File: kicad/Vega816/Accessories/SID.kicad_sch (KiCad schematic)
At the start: 18 parts

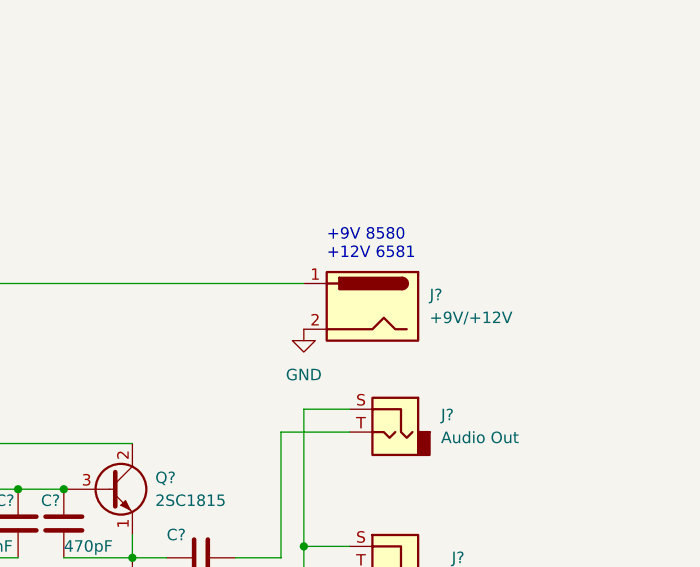
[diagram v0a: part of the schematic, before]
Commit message: Big push, Sysctl, DMA Reg
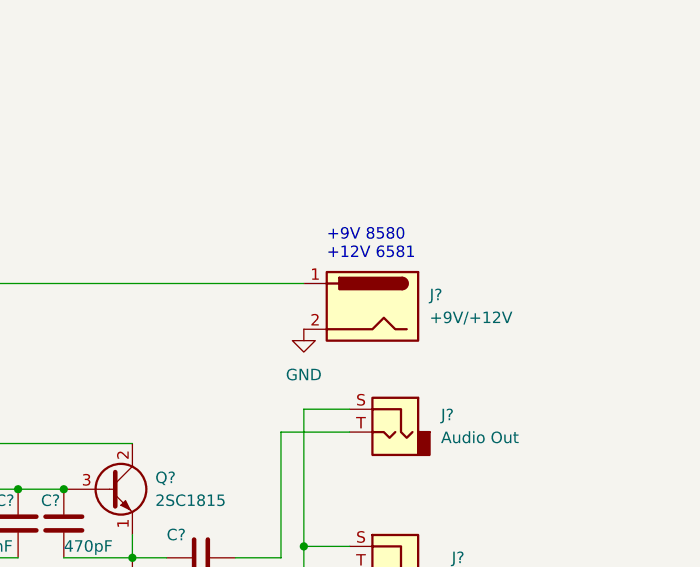
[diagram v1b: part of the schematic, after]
